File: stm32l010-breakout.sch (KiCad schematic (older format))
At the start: 29 parts, among them J1 SWD, J2 Left, J3 Right, Q1 BC847BS, SW1 Reset, U1 STM32L010K8Tx, Y1 32.768kHz

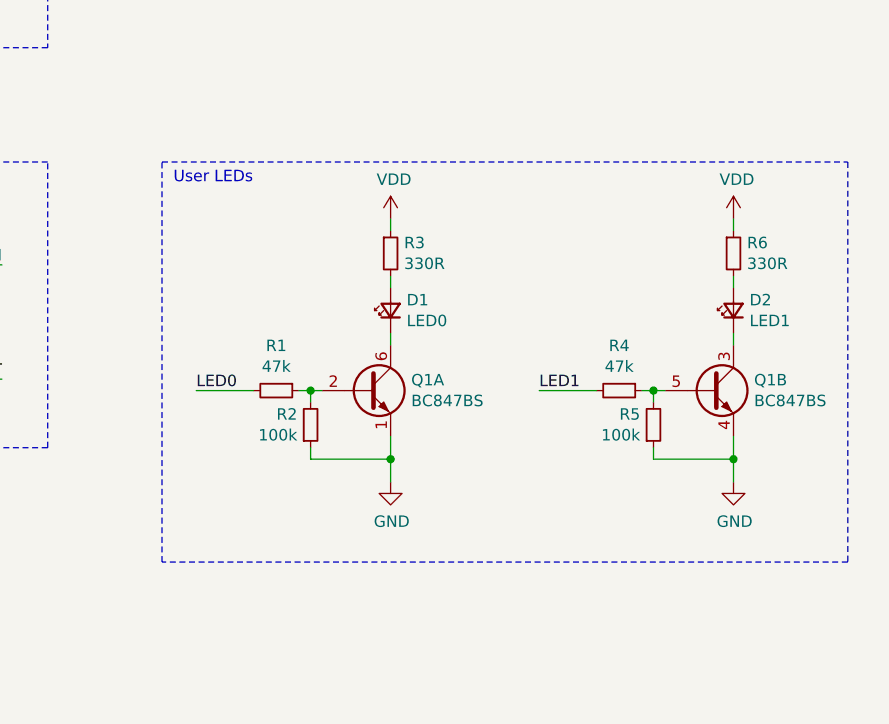
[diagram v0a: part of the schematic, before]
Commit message: Finished laying out Revision B
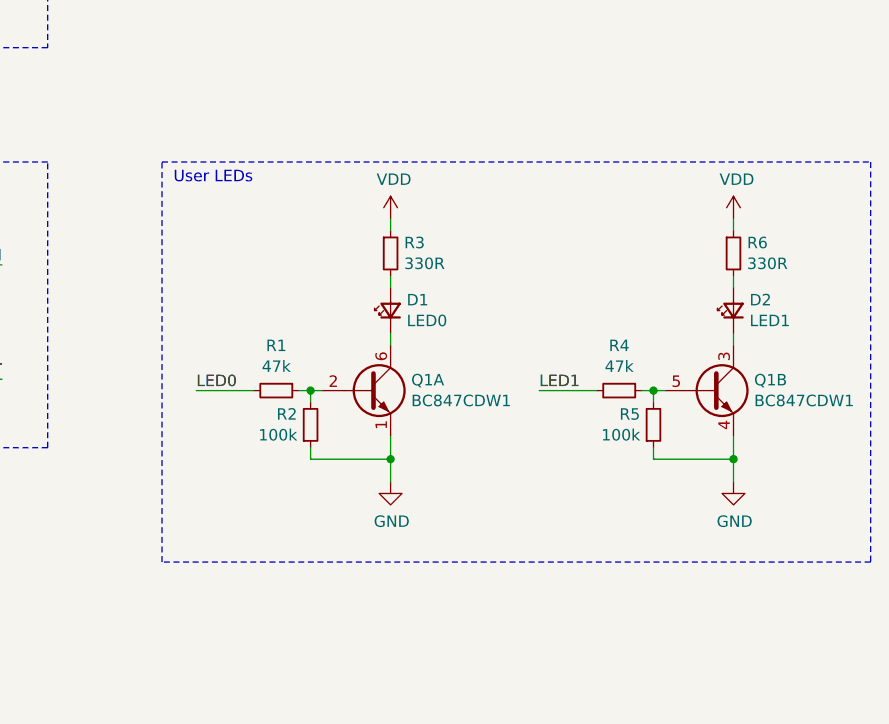
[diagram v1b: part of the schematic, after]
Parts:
- Q1: value BC847BS -> BC847CDW1
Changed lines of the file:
@@
 Sheet 1 1
 Title "STM32L010 Breakout Board"
-Date "2020-07-30"
+Date "2020-08-14"
 Rev "B"
 Comp "Michal Potrzebicz"
-Comment1 "https://creativecommons.org/licenses/by-sa/4.0/"
-Comment2 "Released under the CC BY-SA 4.0 License"
-Comment3 "most of the STM32L0 and STM32L4 chips in LQFP-32 packages"
-Comment4 "Universal STM32L010 breakout board compatible also with"
+Comment1 "other STM32L0 and STM32L4 chips in LQFP-32 packages"
+Comment2 "Universal STM32L010 breakout board compatible also with"
+Comment3 ""
+Comment4 "License: CC BY-SA 4.0"
 $EndDescr
 $Comp
@@
 P 9400 5500
 F 0 "Q1" H 9590 5546 50  0000 L CNN
-F 1 "BC847BS" H 9590 5455 50  0000 L CNN
+F 1 "BC847CDW1" H 9590 5455 50  0000 L CNN
 F 2 "Package_TO_SOT_SMD:SOT-363_SC-70-6" H 9600 5600 50  0001 C CNN
 F 3 "https://assets.nexperia.com/documents/data-sheet/BC847BS.pdf" H 9400 5500 50  0001 C CNN
@@
 P 7900 5500
 F 0 "Q1" H 8090 5546 50  0000 L CNN
-F 1 "BC847BS" H 8090 5455 50  0000 L CNN
+F 1 "BC847CDW1" H 8090 5455 50  0000 L CNN
 F 2 "Package_TO_SOT_SMD:SOT-363_SC-70-6" H 8100 5600 50  0001 C CNN
 F 3 "https://assets.nexperia.com/documents/data-sheet/BC847BS.pdf" H 7900 5500 50  0001 C CNN
@@
 External reset
 Wire Notes Line
-	10000 6250 7000 6250
+	10100 6250 7000 6250
 Wire Notes Line
 	7000 6250 7000 4500
 Wire Notes Line
-	7000 4500 10000 4500
-Wire Notes Line
-	10000 4500 10000 6250
+	7000 4500 10100 4500
+Wire Notes Line
+	10100 4500 10100 6250
 Text Notes 7050 4600 0    50   ~ 0
 User LEDs
